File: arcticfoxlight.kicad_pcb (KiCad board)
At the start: 2 copper layers, 41.5 x 44 mm, 22 parts, among them J1 USB_C_Receptacle_USB2.0_16P, SW1 RESET, SW2 FLASH, U1 LM2596S-5, U2 ESP32-C6-MINI-1/U, U3 LM2596S-3.3, U4 SN74AHCT125N

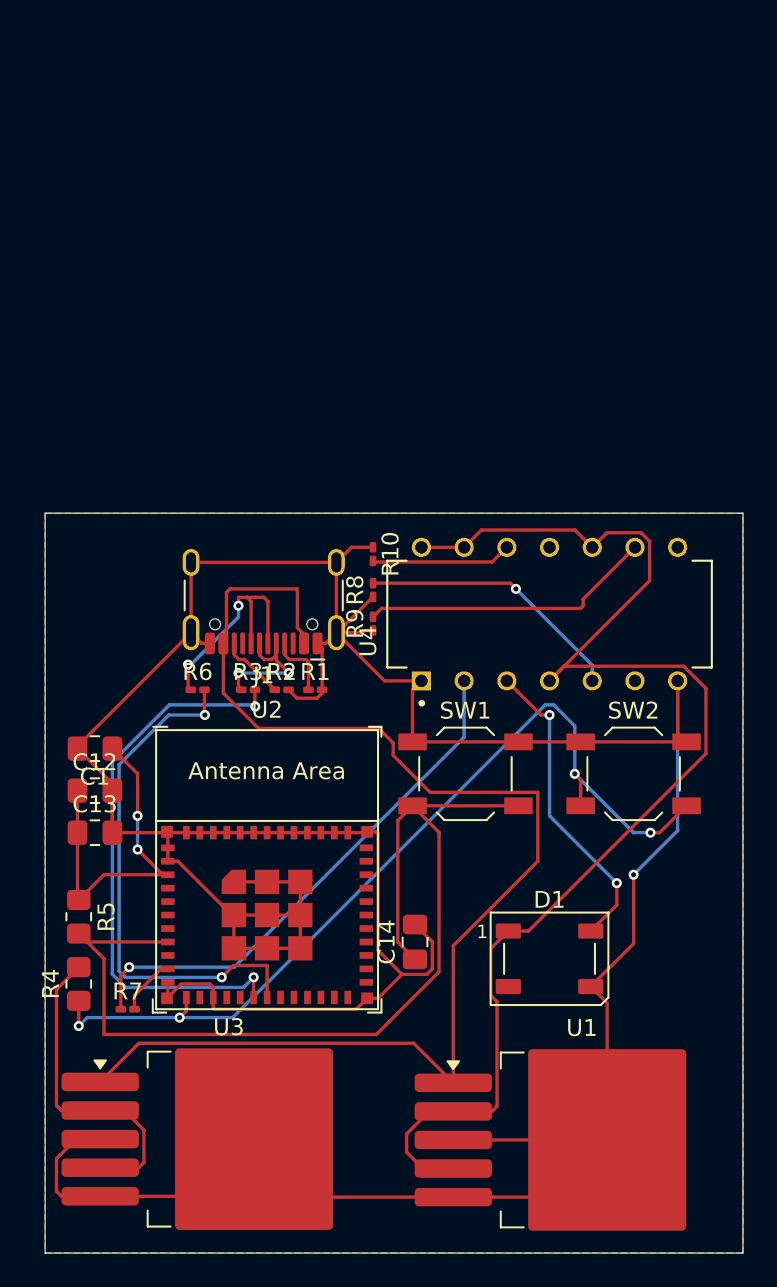
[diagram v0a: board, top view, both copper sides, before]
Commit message: Day 2.1
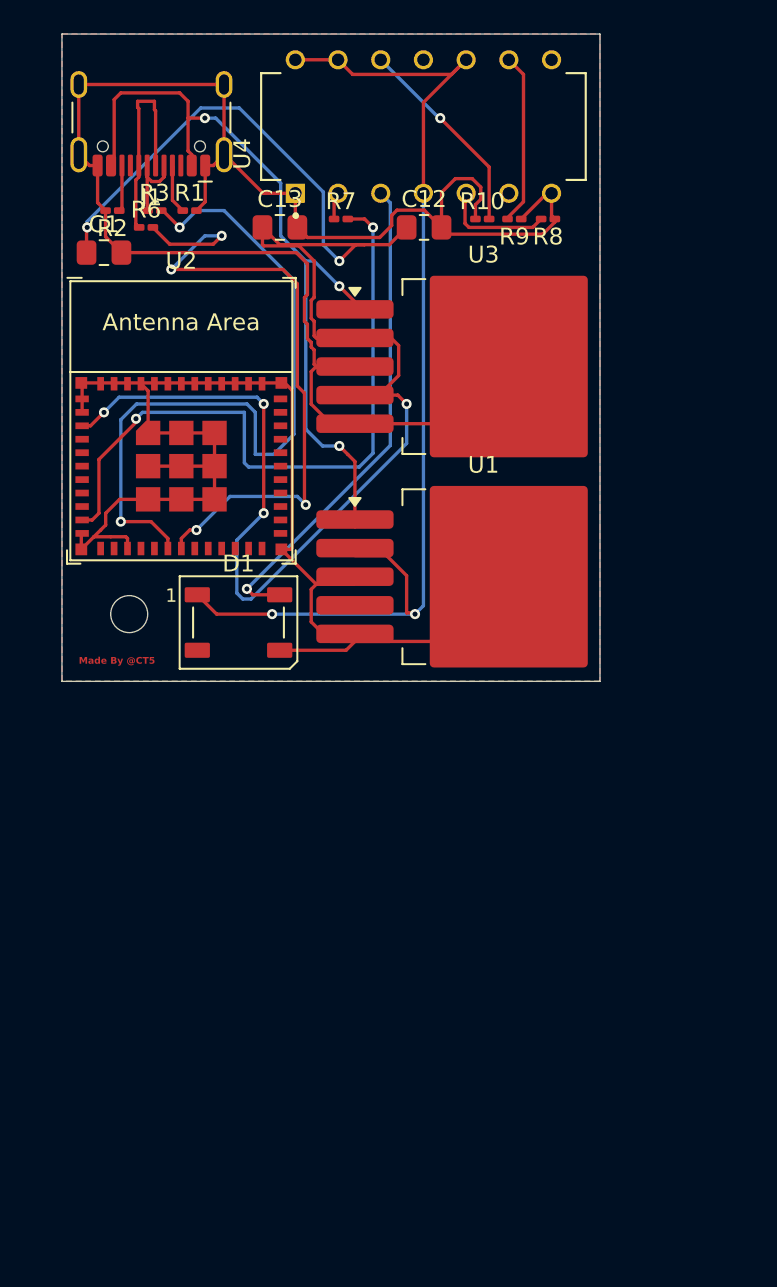
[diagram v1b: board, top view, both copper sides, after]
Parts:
- removed C14: 100nF, Capacitor_SMD:C_0805_2012Metric_Pad1.18x1.45mm_HandSolder
- removed R4, R5: 10k, Resistor_SMD:R_0805_2012Metric_Pad1.20x1.40mm_HandSolder
- removed SW1: RESET, Button_Switch_SMD:SW_SPST_TL3342
- removed SW2: FLASH, Button_Switch_SMD:SW_SPST_TL3342
- added H1: MountingHole, MountingHole:MountingHole_2.2mm_M2, F.Cu at (22.5, 79.5)
- moved R7 48.7 mm to (35.1, 56.0)
- moved U3 48.4 mm to (43.6, 64.8)
- moved C12 38.8 mm to (40.0, 56.5)
- moved C13 37.6 mm to (31.5, 56.5)
- moved U1 34.0 mm to (43.6, 77.3)
- moved R2 30.2 mm to (21.5, 55.5), turned to 180 degrees
- moved U4 30.0 mm to (40.0, 50.5)
- moved C1 29.5 mm to (21.0, 58.0), turned to 0 degrees
- moved R1 29.5 mm to (26.1, 55.5)
- moved J1 29.2 mm to (23.8, 49.1)
- moved R3 29.0 mm to (24.0, 55.5)
- moved R6 27.7 mm to (23.5, 56.5)
- moved D1 27.2 mm to (29.0, 80.0)
- moved U2 27.2 mm to (25.6, 68.0)
- moved R9 25.5 mm to (45.4, 56.0), turned to 180 degrees
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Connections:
- U2 pad 12: BOOT -> unconnected-(U2-GPIO0/ADC1_CH0/XTAL_32K_P-Pad12)
- U2 pad 8: EN -> unconnected-(U2-EN/CHIP_PU-Pad8)
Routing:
- net EN: track 60.4 -> 0.00 mm
- net +3.3V: track 40.7 -> 99.1 mm, vias 2 -> 6
- net BOOT: track 54.5 -> 0.00 mm, vias 4 -> 0
- net GND: track 232.6 -> 179.1 mm, vias 1 -> 0
- net Net-(U2-MTDI/GPIO5/ADC1_CH5): track 3.46 -> 40.5 mm, vias 0 -> 2
- net VCC: track 77.6 -> 47.0 mm, vias 0 -> 3
- net DIN: track 31.6 -> 1.63 mm, vias 1 -> 0
- net +5V: track 77.3 -> 64.8 mm, vias 0 -> 2
- net Net-(D1-DIN): track 18.5 -> 29.4 mm, vias 2 -> 1
- net D-: track 33.8 -> 43.4 mm
- net Net-(U4-2A): track 16.0 -> 6.66 mm, vias 1 -> 0
- net D+: track 31.3 -> 39.0 mm, vias 2 -> 4
- net Net-(U4-3A): track 17.5 -> 10.2 mm
- net Net-(U4-4A): track 8.35 -> 12.2 mm, vias 0 -> 1
- net Net-(J1-D--PadA7): track 8.72 -> 5.28 mm, vias 2 -> 0
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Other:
- board size 41.5 x 44 mm -> 32 x 38.5 mm
